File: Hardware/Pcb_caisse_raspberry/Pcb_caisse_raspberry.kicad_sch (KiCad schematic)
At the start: 24 parts, among them J1 Conn_02x20_Odd_Even, J2 Conn_01x04, J3 Conn_01x08, J5 Conn_01x08

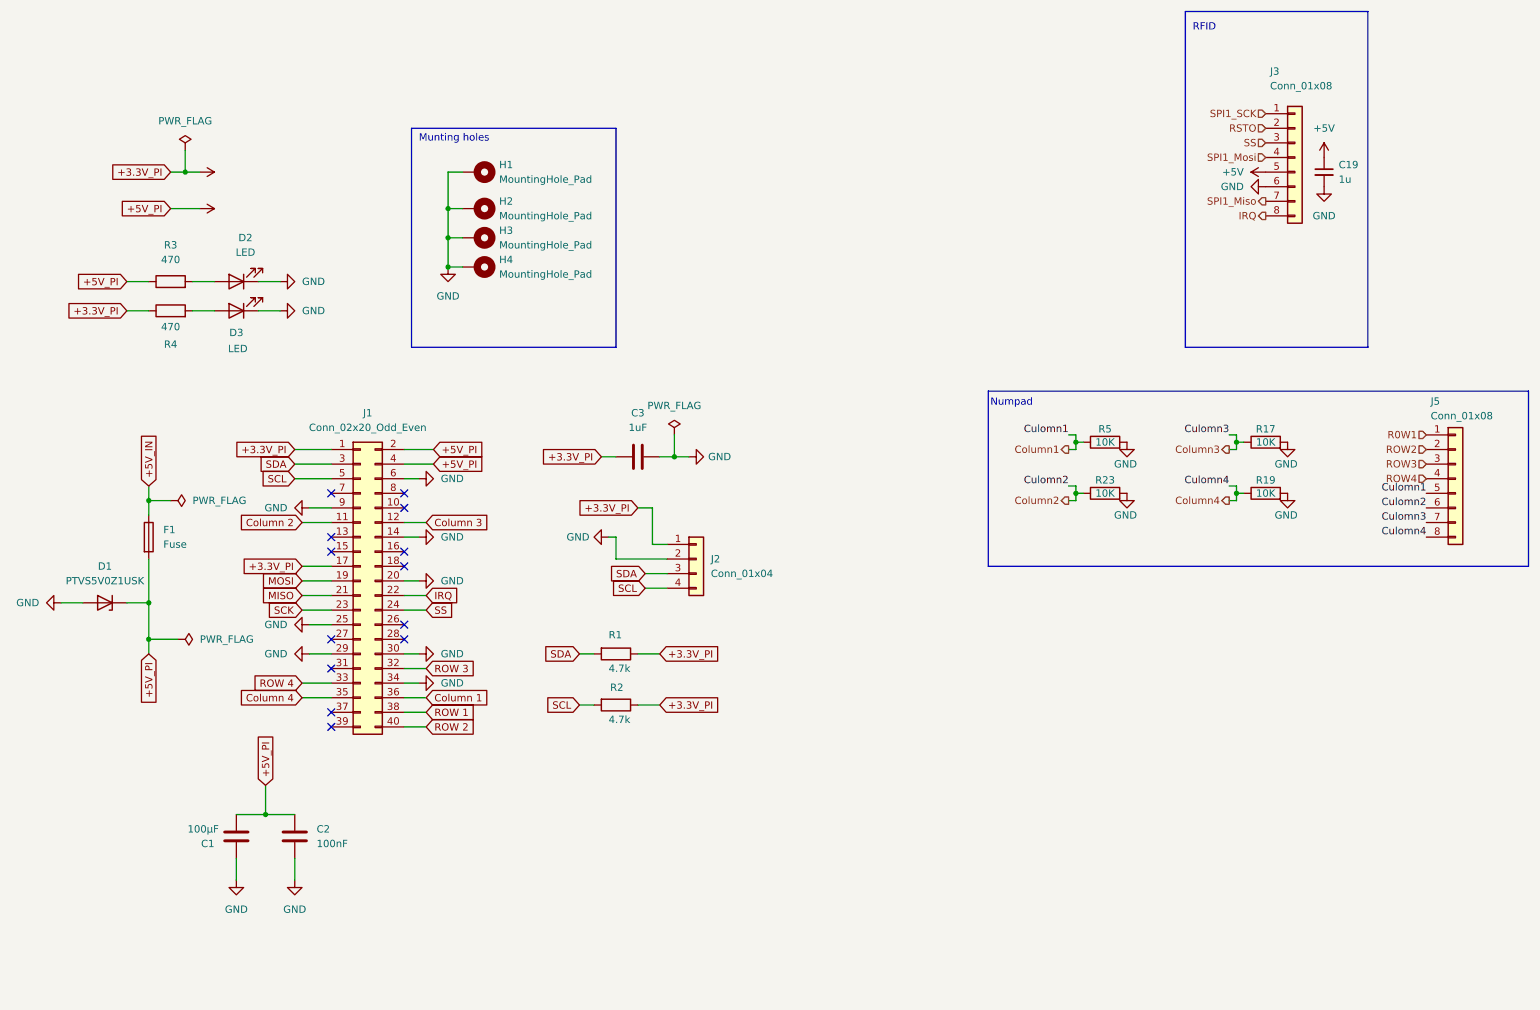
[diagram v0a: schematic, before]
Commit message: Add files via upload
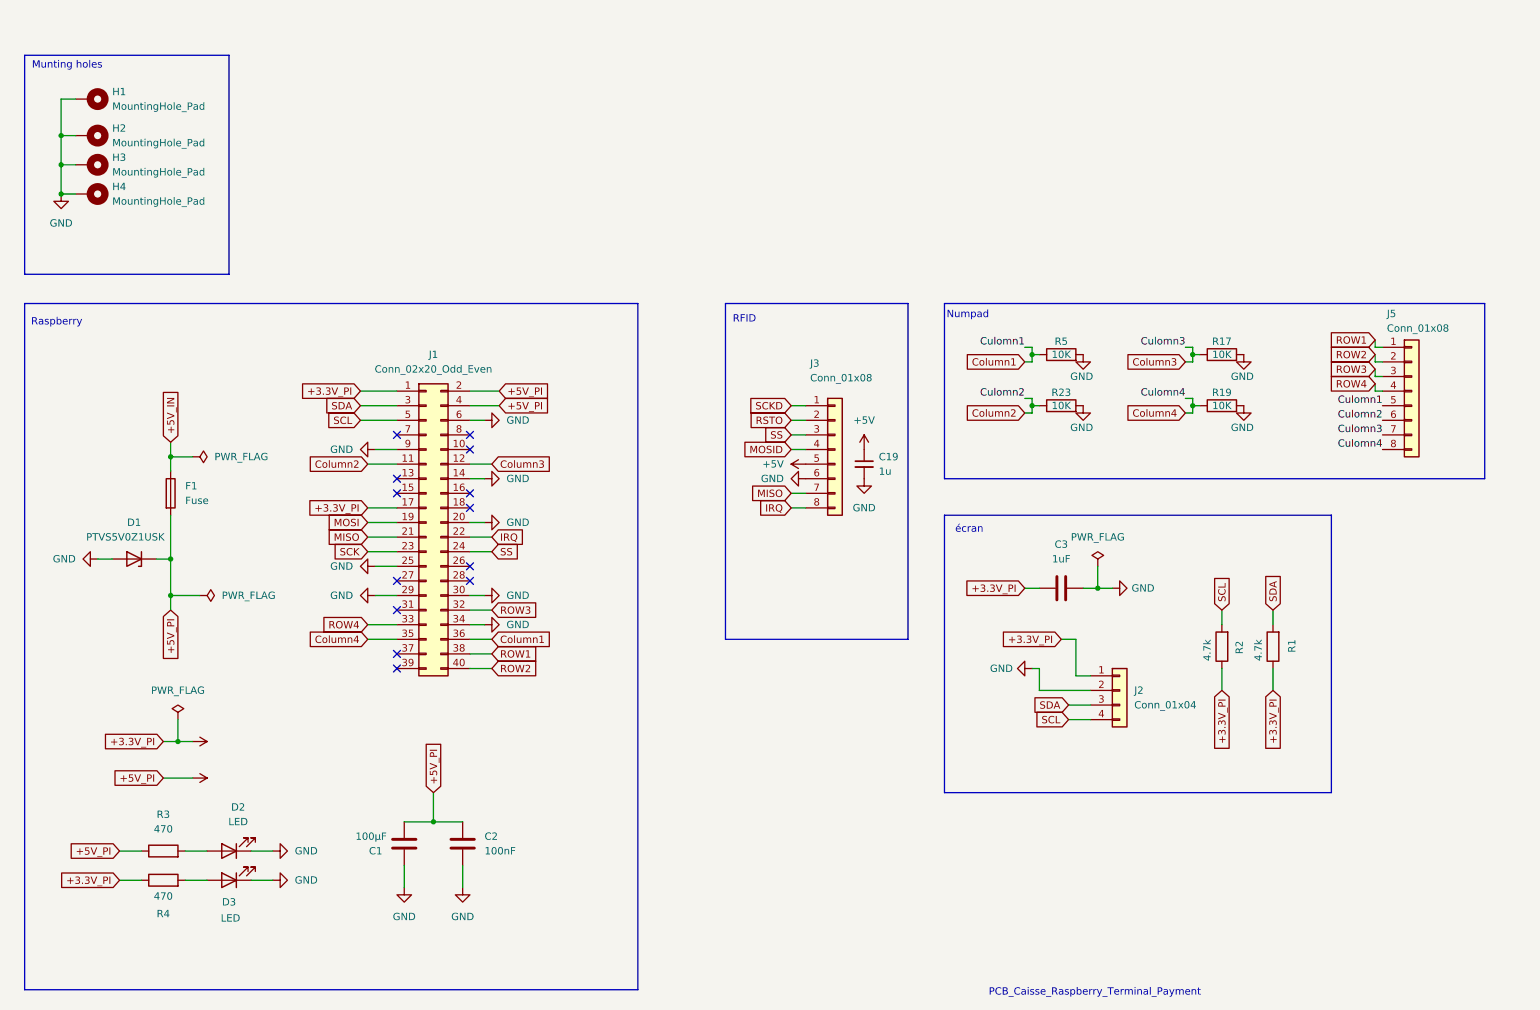
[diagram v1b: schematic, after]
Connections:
- net Column 1 is gone; now on net Column1: J1.36 (Pin_36)
- net Column 2 is gone; now on net Column2: J1.11 (Pin_11)
- net Column 3 is gone; now on net Column3: J1.12 (Pin_12)
- net Column 4 is gone; now on net Column4: J1.35 (Pin_35)
- net ROW 1 is gone; now on net ROW1: J1.38 (Pin_38)
- net ROW 2 is gone; now on net ROW2: J1.40 (Pin_40)
- net ROW 3 is gone; now on net ROW3: J1.32 (Pin_32)
- net ROW 4 is gone; now on net ROW4: J1.33 (Pin_33)
- net SPI1_Miso is gone; now on net MISO: J3.7 (Pin_7)
- net R0W1 renamed ROW1
- net SPI1_Mosi renamed MOSID
- net SPI1_SCK renamed SCKD
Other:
- note added: "PCB_Caisse_Raspberry_Terminal_Payment"
- note added: "Raspberry"
- note added: "écran"
- moved on the sheet: C1, C19, C2, C3, D1, D2, D3, F1, H1, H2, H3, H4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

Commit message: Add files via upload
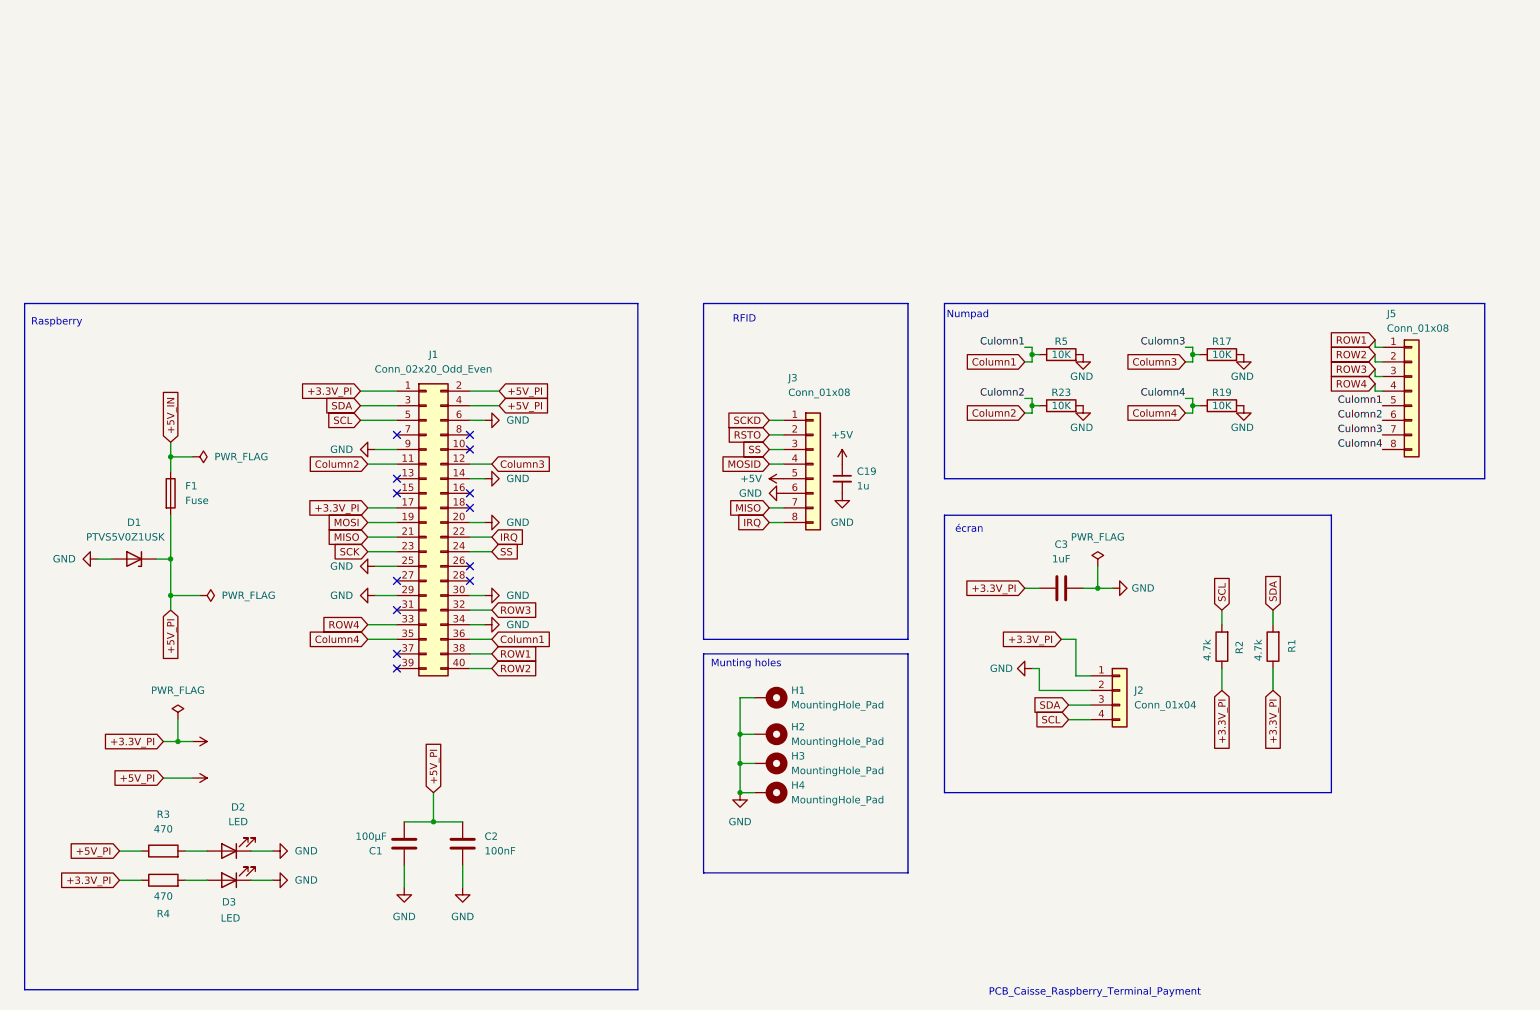
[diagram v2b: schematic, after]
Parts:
- C1, C2, C3: footprint (none) -> Capacitor_SMD:C_0603_1608Metric_Pad1.08x0.95mm_HandSolder
- C19: footprint Capacitor_SMD:C_0402_1005Metric -> Capacitor_SMD:C_0603_1608Metric_Pad1.08x0.95mm_HandSolder
- D2, D3: footprint (none) -> LED_SMD:LED_0603_1608Metric_Pad1.05x0.95mm_HandSolder
- F1: footprint (none) -> Fuse:FuseHolder_Blade_ATO_Littelfuse_FLR_178.6165
- J1: footprint (none) -> Connector_PinHeader_1.00mm:PinHeader_2x20_P1.00mm_Vertical
- J2: footprint (none) -> Connector_PinHeader_2.54mm:PinHeader_1x04_P2.54mm_Horizontal
- R1, R2, R3, R4: footprint (none) -> Resistor_SMD:R_0603_1608Metric_Pad0.98x0.95mm_HandSolder
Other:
- moved on the sheet: C19, H1, H2, H3, H4, J3
